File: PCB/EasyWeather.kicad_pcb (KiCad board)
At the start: 2 copper layers, 31.5 x 55.5 mm, 5 parts, among them U1 BME280-3.3V Module, U2 XIAO-ESP32-S3-DIP, U3 SSD1306

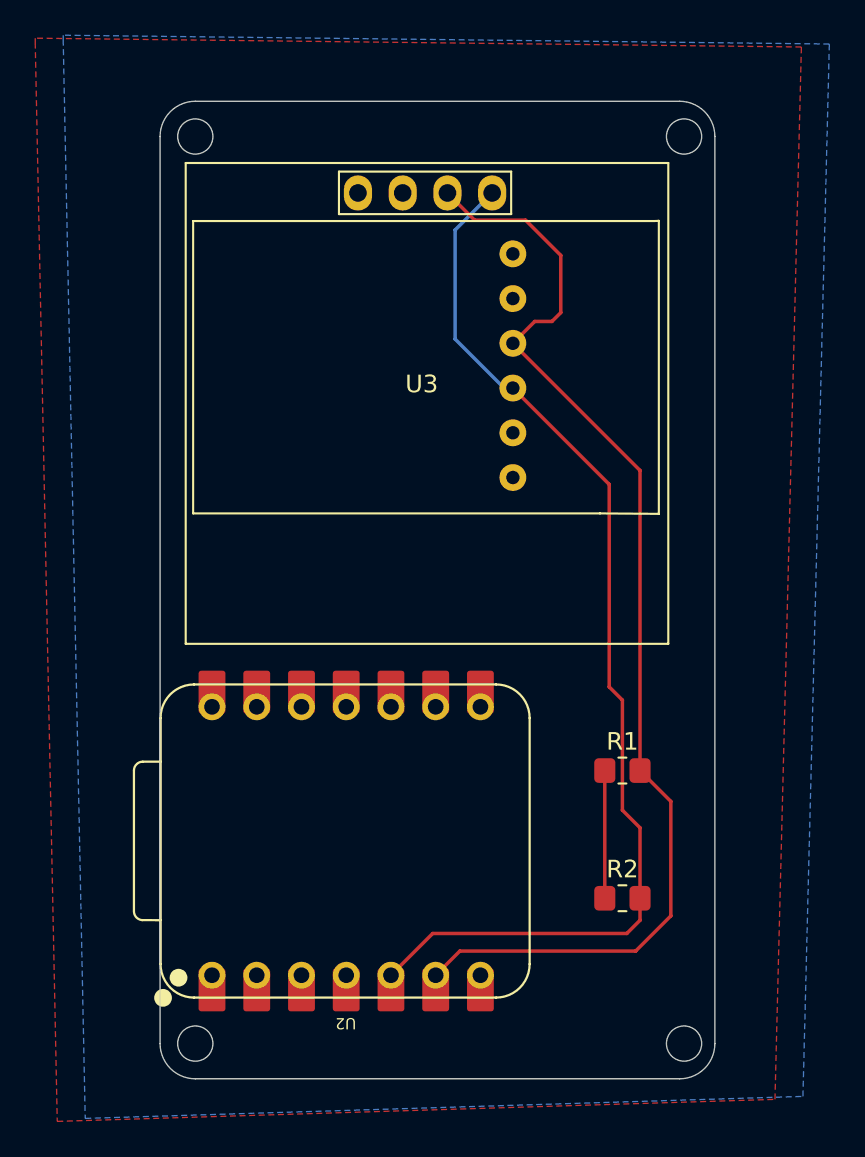
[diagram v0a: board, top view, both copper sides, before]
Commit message: CAD
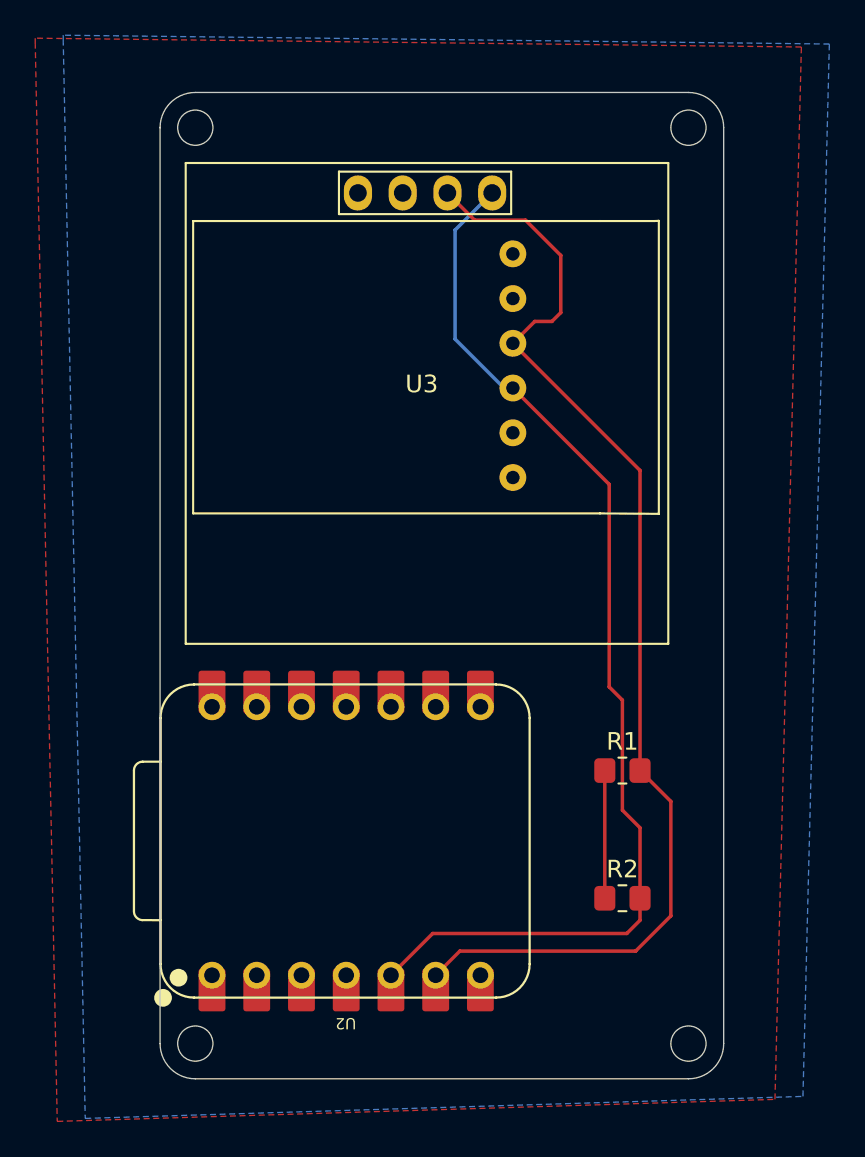
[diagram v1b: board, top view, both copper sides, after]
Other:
- board size 31.5 x 55.5 mm -> 32 x 56 mm
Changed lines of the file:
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@@
 		)
 	)
-	(gr_line
-		(start 118 98)
-		(end 118 46.5)
-		(stroke
-			(width 0.05)
-			(type default)
-		)
-		(layer "Edge.Cuts")
-	)
-	(gr_line
-		(start 149.5 46.5)
-		(end 149.5 98)
+	(gr_arc
+		(start 118 46)
+		(mid 118.585786 44.585786)
+		(end 120 44)
 		(stroke
 			(width 0.05)
@@
 	)
 	(gr_arc
-		(start 147.5 44.5)
-		(mid 148.914214 45.085786)
-		(end 149.5 46.5)
+		(start 148 44)
+		(mid 149.414214 44.585786)
+		(end 150 46)
+		(stroke
+			(width 0.05)
+			(type default)
+		)
+		(layer "Edge.Cuts")
+	)
+	(gr_arc
+		(start 150 98)
+		(mid 149.414214 99.414214)
+		(end 148 100)
 		(stroke
 			(width 0.05)
@@
 	)
 	(gr_circle
-		(center 120 46.5)
-		(end 121 46.5)
+		(center 120 46)
+		(end 121 46)
 		(stroke
 			(width 0.05)
@@
 		(layer "Edge.Cuts")
 	)
-	(gr_line
-		(start 147.5 100)
-		(end 120 100)
-		(stroke
-			(width 0.05)
-			(type default)
-		)
-		(layer "Edge.Cuts")
-	)
-	(gr_arc
-		(start 118 46.5)
-		(mid 118.585786 45.085786)
-		(end 120 44.5)
-		(stroke
-			(width 0.05)
-			(type default)
-		)
-		(layer "Edge.Cuts")
-	)
 	(gr_circle
-		(center 147.75 98)
-		(end 148.75 98)
+		(center 148 98)
+		(end 149 98)
 		(stroke
 			(width 0.05)
@@
 	)
 	(gr_line
-		(start 120 44.5)
-		(end 147.5 44.5)
+		(start 120 44)
+		(end 148 44)
+		(stroke
+			(width 0.05)
+			(type default)
+		)
+		(layer "Edge.Cuts")
+	)
+	(gr_line
+		(start 150 46)
+		(end 150 98)
 		(stroke
 			(width 0.05)
@@
 		(layer "Edge.Cuts")
 	)
-	(gr_arc
-		(start 149.5 98)
-		(mid 148.914214 99.414214)
-		(end 147.5 100)
+	(gr_line
+		(start 148 100)
+		(end 120 100)
+		(stroke
+			(width 0.05)
+			(type default)
+		)
+		(layer "Edge.Cuts")
+	)
+	(gr_line
+		(start 118 98)
+		(end 118 46)
 		(stroke
 			(width 0.05)
@@
 	)
 	(gr_circle
-		(center 147.75 46.5)
-		(end 148.75 46.5)
+		(center 148 46)
+		(end 149 46)
 		(stroke
 			(width 0.05)
